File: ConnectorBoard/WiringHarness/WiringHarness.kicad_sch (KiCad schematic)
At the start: 15 parts, among them J1 Barrel_Jack, J2 Conn_01x03, J3 Conn_01x03, J4 Conn_02x05_Odd_Even, U1 L7805, U2 L7805

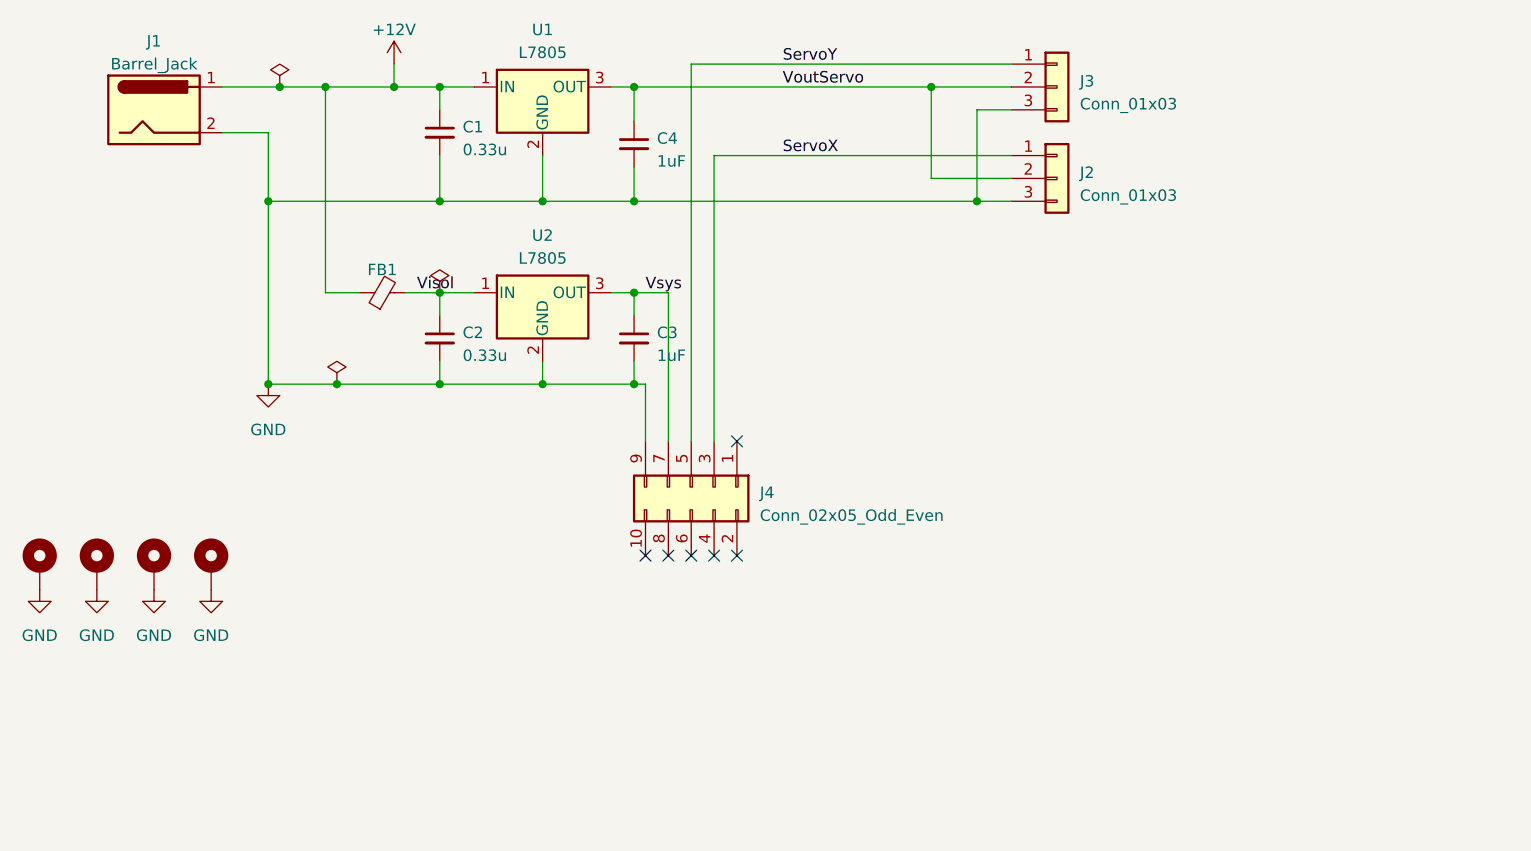
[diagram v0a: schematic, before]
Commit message: updates to connector
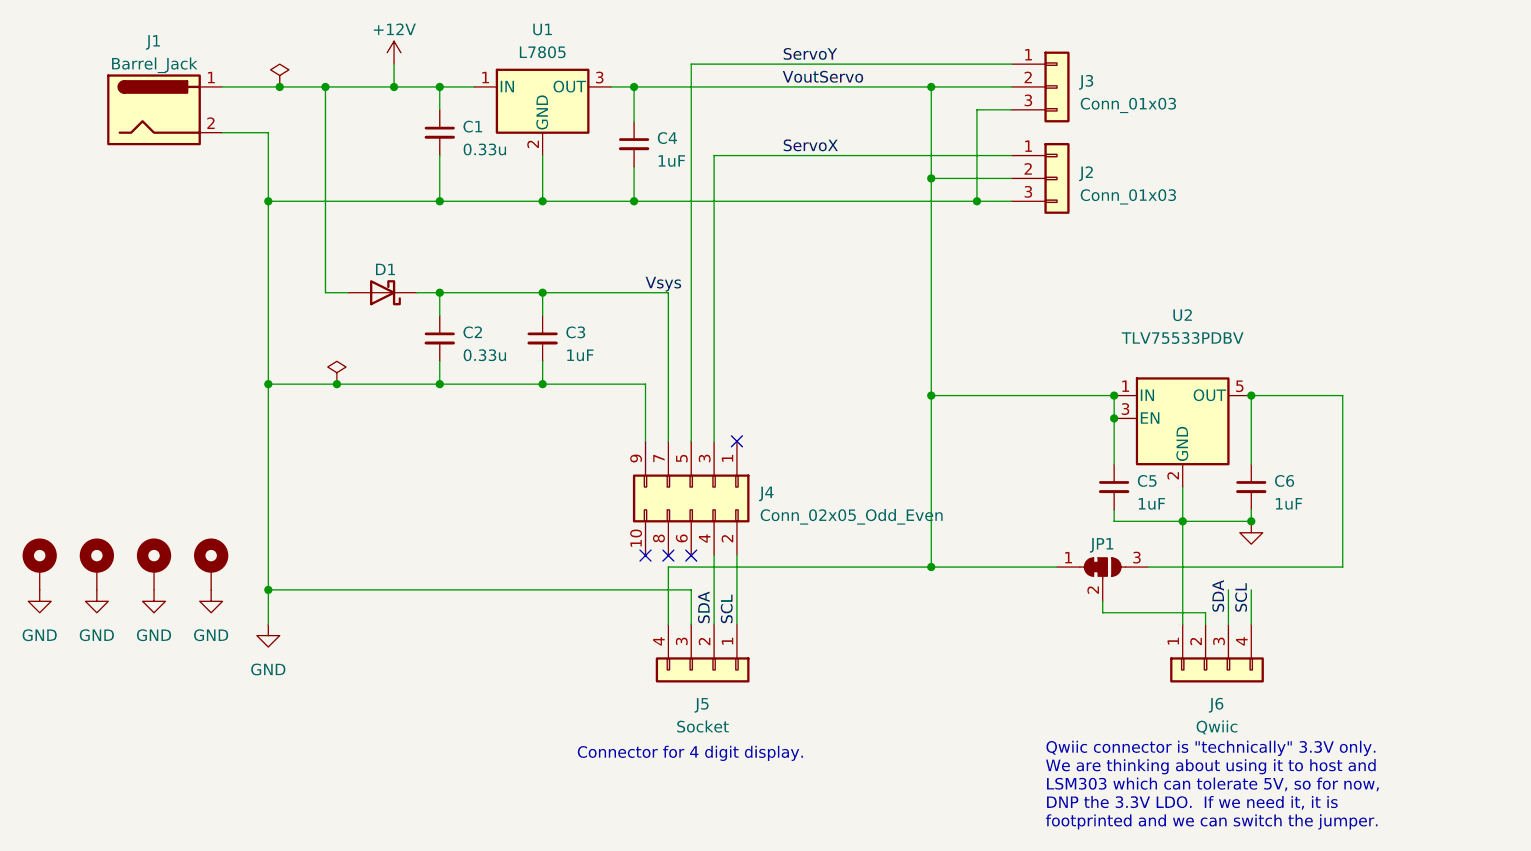
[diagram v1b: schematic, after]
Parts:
- removed FB1: FerriteBead_Small, Inductor_SMD:L_0603_1608Metric, symbol Device:FerriteBead_Small
- removed U2: L7805, Package_TO_SOT_SMD:TO-252-2, symbol Regulator_Linear:L7805
- added C5, C6: 1uF, Capacitor_SMD:C_0603_1608Metric, symbol Device:C_Small
- added D1: D_Schottky, Diode_SMD:D_SMA, symbol Device:D_Schottky
- added J5: Socket, Connector_PinSocket_2.54mm:PinSocket_1x04_P2.54mm_Vertical, symbol Connector_Generic:Conn_01x04
- added J6: Qwiic, Connector_JST:JST_SH_SM04B-SRSS-TB_1x04-1MP_P1.00mm_Horizontal, symbol Connector_Generic:Conn_01x04
- added JP1: SolderJumper_3_Bridged12, Jumper:SolderJumper-3_P1.3mm_Bridged12_RoundedPad1.0x1.5mm, symbol Jumper:SolderJumper_3_Bridged12
- added U2: TLV75533PDBV, Package_TO_SOT_SMD:SOT-23-5, symbol Regulator_Linear:TLV75533PDBV
- J2, J3: footprint Connector_PinHeader_1.00mm:PinHeader_1x03_P1.00mm_Horizontal -> Connector_PinHeader_2.54mm:PinHeader_1x03_P2.54mm_Horizontal
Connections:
- net Visol is gone; now on net Vsys: C2.1
- net +12V: now also D1.2 (A)
- net GND: now also C5.2, C6.2, J5.3 (Pin_3), J6.1 (Pin_1), U2.2 (GND)
- net VoutServo: now also C5.1, J5.4 (Pin_4), JP1.1 (A), U2.1 (IN), U2.3 (EN)
- net Vsys: now also D1.1 (K)
- net SCL: now reaches J4.2 (Pin_2)
- net SCL: now also J5.1 (Pin_1), J6.4 (Pin_4)
- net SDA: now reaches J4.4 (Pin_4)
- net SDA: now also J5.2 (Pin_2), J6.3 (Pin_3)
- new net: C6.1, JP1.3 (B), U2.5 (OUT)
- new net: J6.2 (Pin_2), JP1.2 (C)
- no-connect marks 6 -> 4
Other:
- note added: "Connector for 4 digit display."
- note added: "Qwiic connector is "technically" 3.3V only. We are thinking about using it to host and LSM303 which can tolerate 5V, so for now, DNP the 3.3V LDO. If we need it, it is footprinted and we can switch the jumper."
- moved on the sheet: C3

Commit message: decent candidate for rev 0.5wh
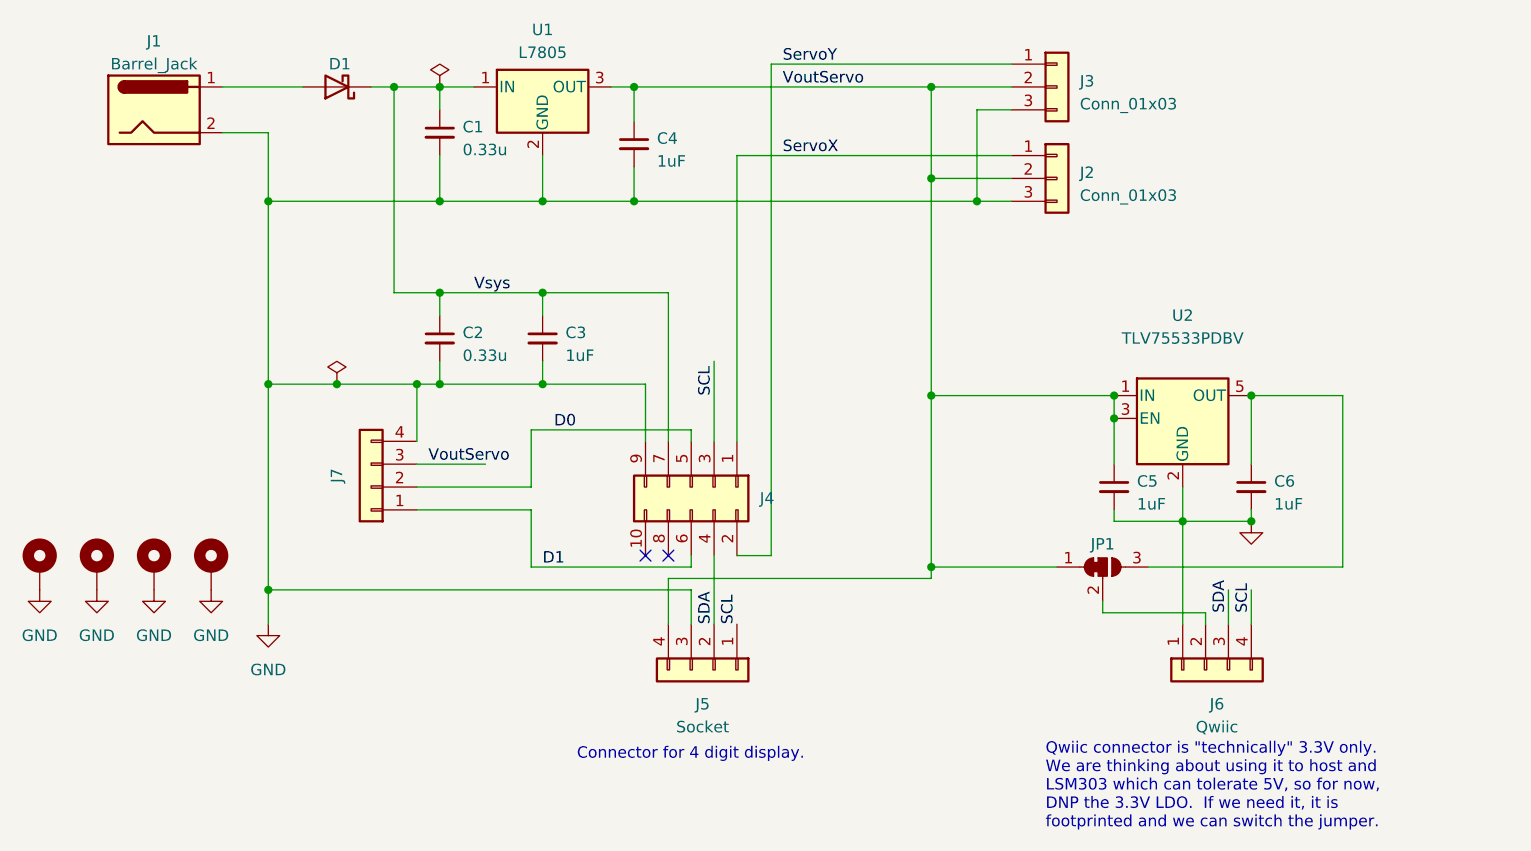
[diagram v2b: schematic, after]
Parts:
- added J7: Header, Connector_PinHeader_2.54mm:PinHeader_1x04_P2.54mm_Horizontal, symbol Connector_Generic:Conn_01x04
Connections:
- net GND: now also J7.4 (Pin_4)
- net SCL: now also J4.3 (Pin_3); no longer J4.2 (Pin_2)
- net ServoX: now also J4.1 (Pin_1); no longer J4.3 (Pin_3)
- net ServoY: now also J4.2 (Pin_2); no longer J4.5 (Pin_5)
- net VoutServo: now also J7.3 (Pin_3)
- net Vsys: now also C1.1, U1.1 (IN)
- net D1: now reaches J4.6 (Pin_6)
- net D1: now also J7.1 (Pin_1)
- net +12V: no longer names the net of D1.2 (A), J1.1
- net +12V: no longer C1.1, U1.1 (IN)
- new net D0: J4.5 (Pin_5), J7.2 (Pin_2)
- no-connect marks 4 -> 2
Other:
- moved on the sheet: D1
